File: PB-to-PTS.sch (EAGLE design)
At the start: 4 parts, among them J1 PulseBlaster, J3 PTS-PORT

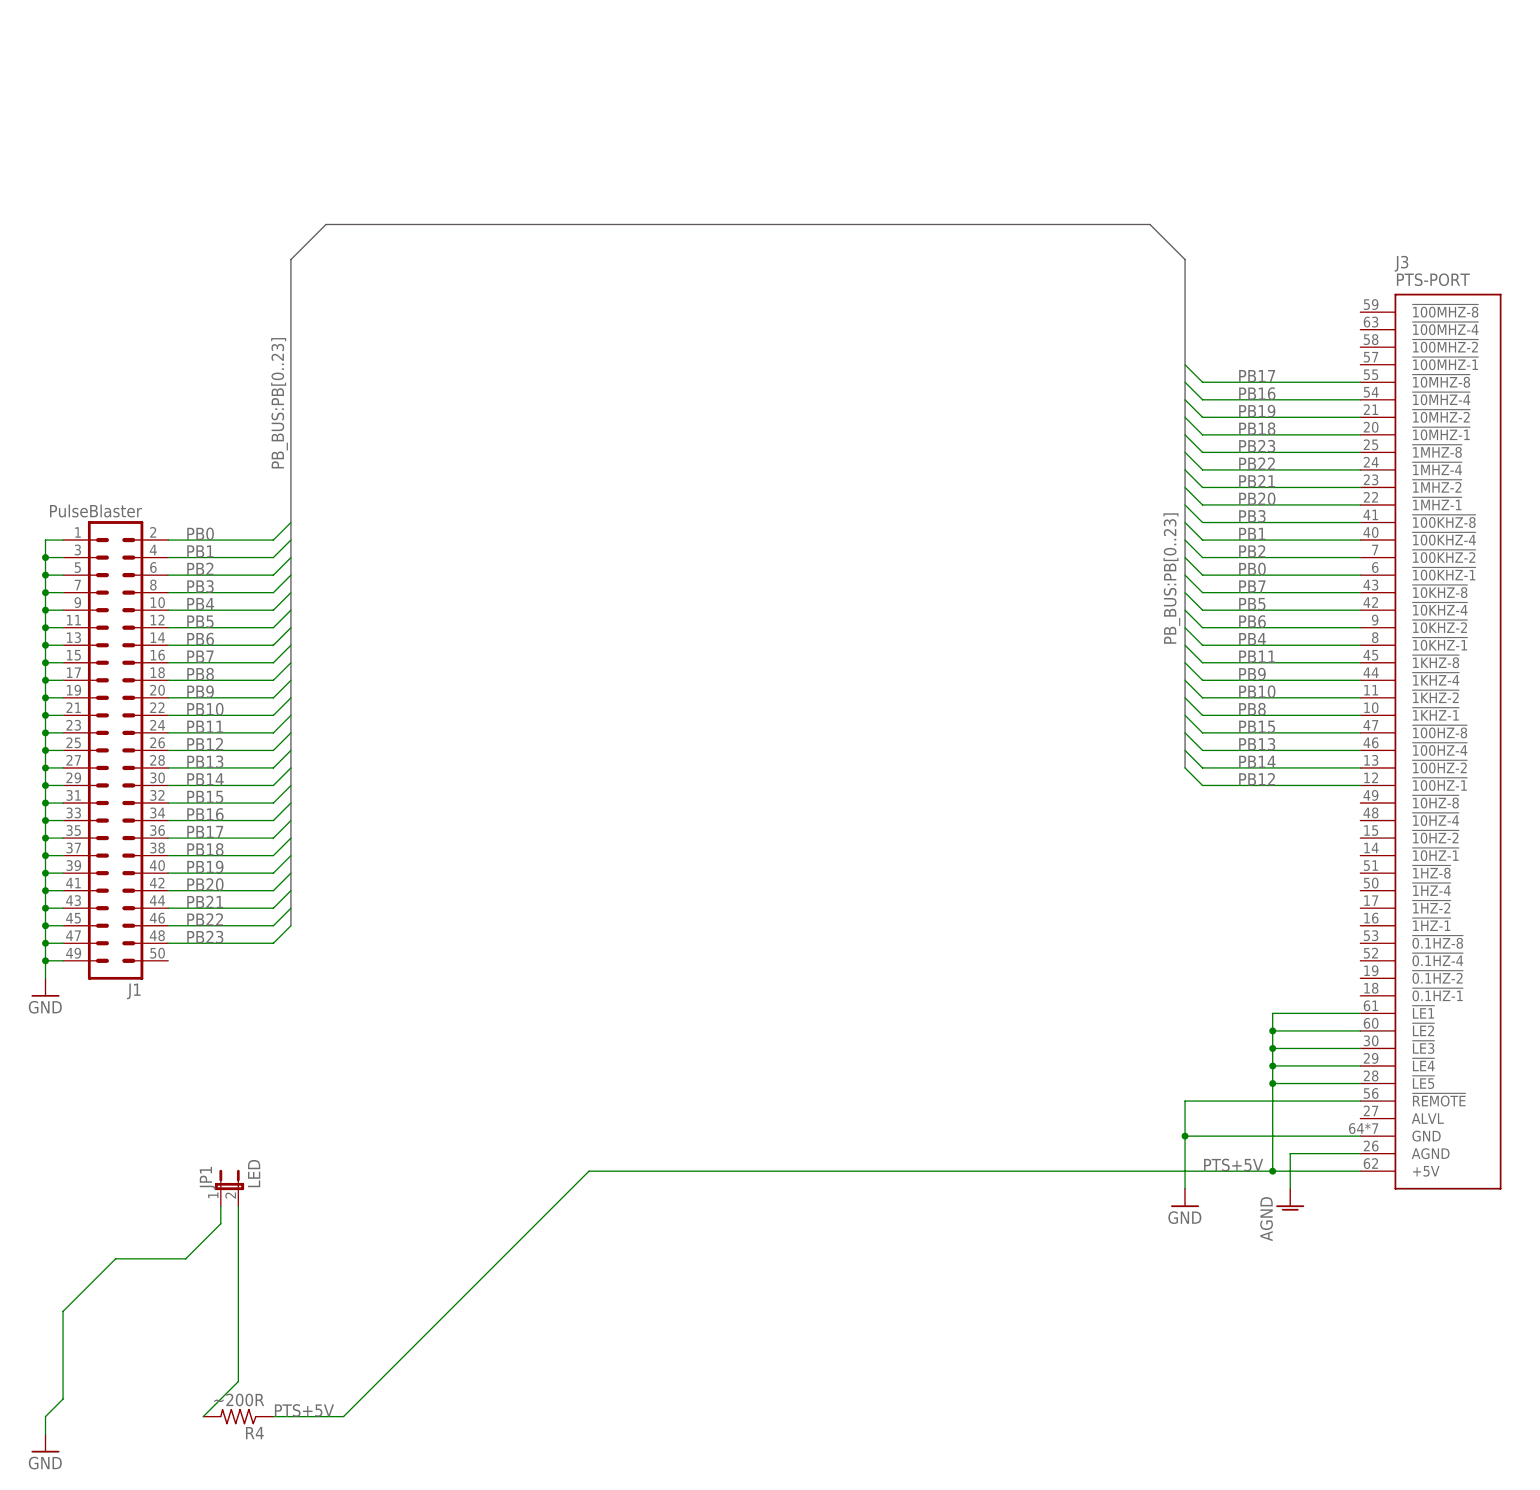
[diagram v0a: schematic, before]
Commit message: Clean up schematic, route board
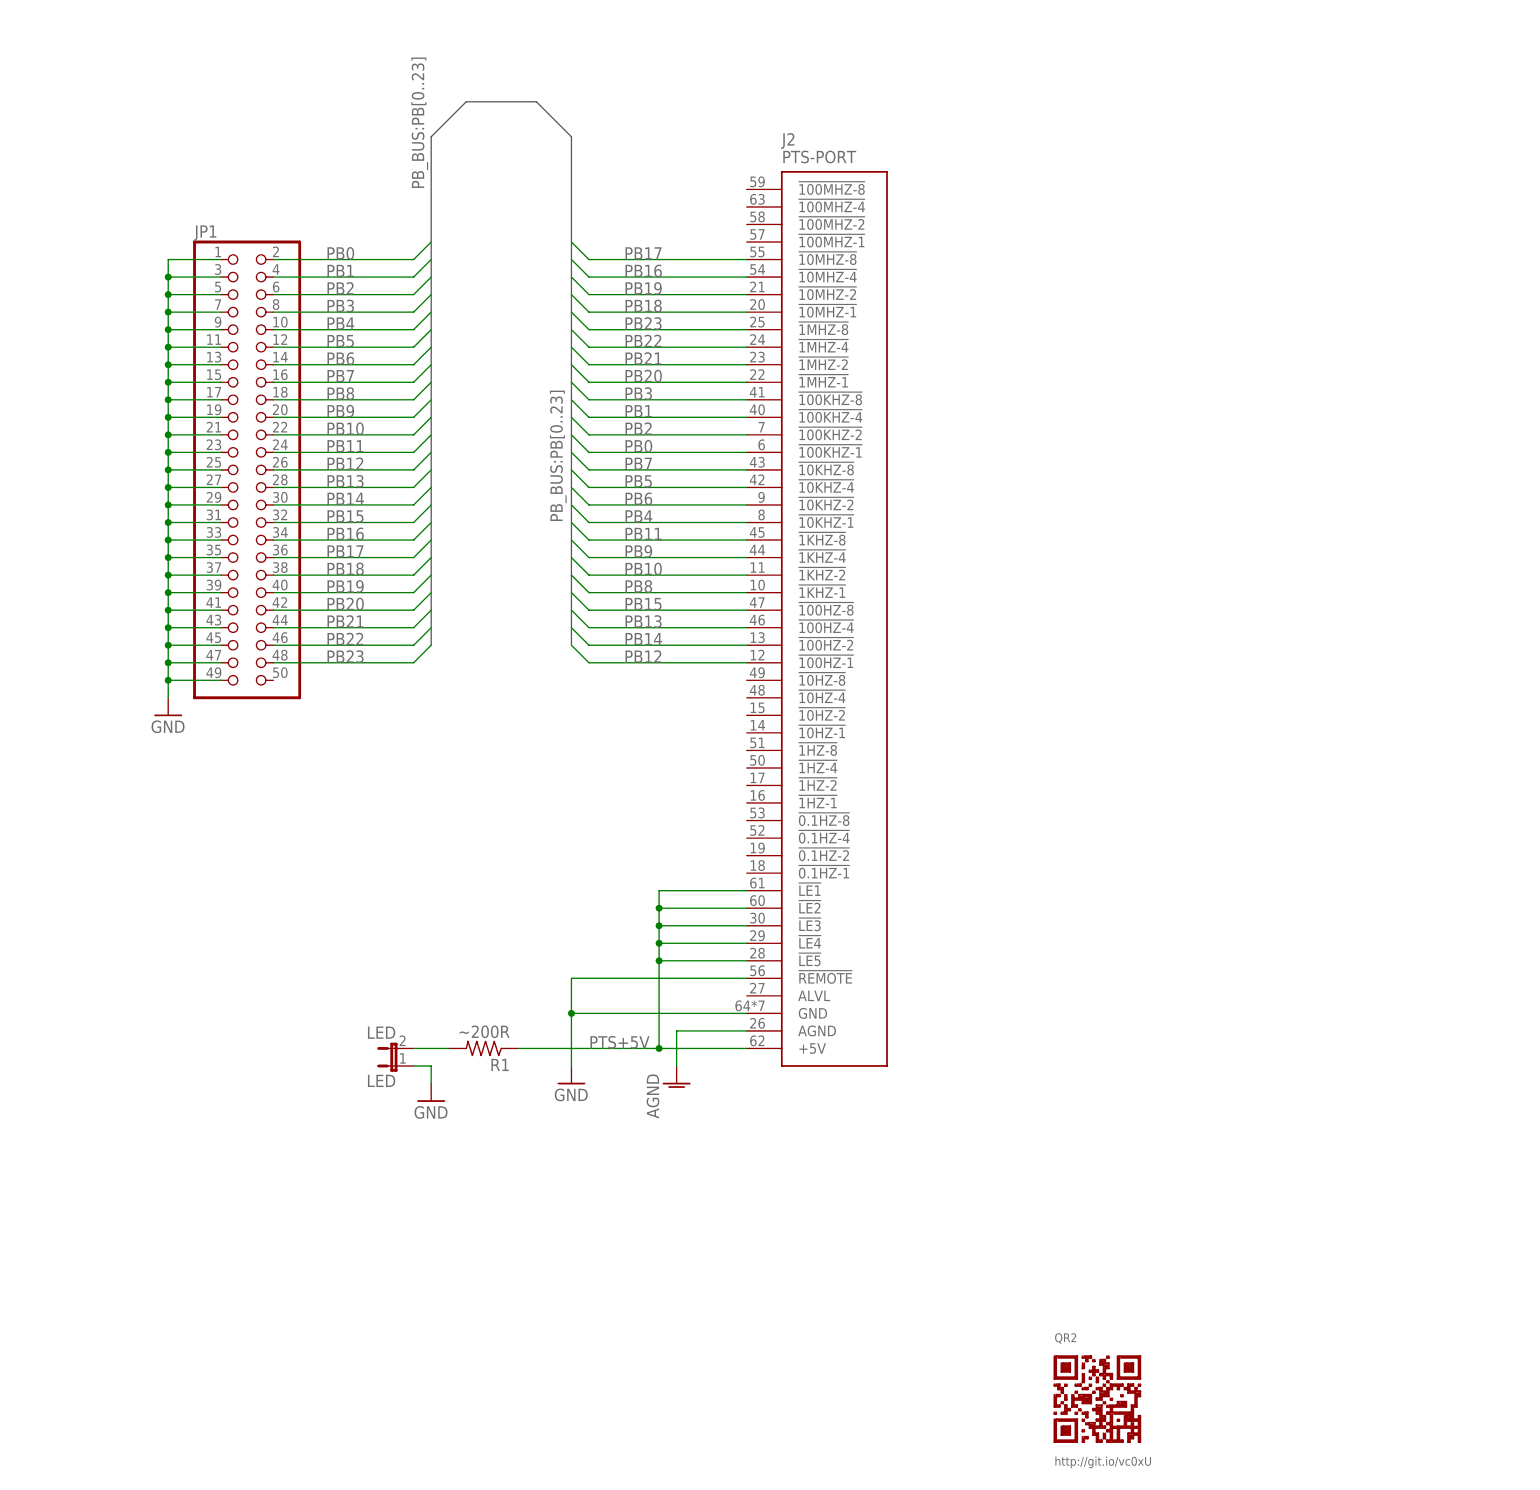
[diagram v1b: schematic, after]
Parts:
- removed J1: PulseBlaster, PTS_Board_Lib:HARTING-09185505909
- removed J3: PTS-PORT, PTS_Board_Lib:PTS-PORT
- removed R4: ~200R, resistor:R-US_R1206
- added J2: PTS-PORT, PTS_Board_Lib:PTS-PORT
- added LED: LED, jumper:JP1E
- added QR2: QR-HTTP://GIT.IO/VC0XU, QR-git.io-vc0xU:QR-HTTP://GIT.IO/VC0XU
- added R1: ~200R, resistor:R-US_R0805
- JP1: value LED -> (none); device jumper:JP1E -> pinhead:PINHD-2X25
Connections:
- net AGND: now also J2.AGND; no longer J3.AGND
- net GND: now also J2.!REMOTE, J2.GND, JP1.11, JP1.13, JP1.15, JP1.17, JP1.19, JP1.21, JP1.23, JP1.25, JP1.27, JP1.29, JP1.3, JP1.31, JP1.33, JP1.35, JP1.37, JP1.39, JP1.41, JP1.43, JP1.45, JP1.47, JP1.49, JP1.5, JP1.7, JP1.9, LED.1; no longer J1.1, J1.11, J1.13, J1.15, J1.17, J1.19, J1.21, J1.23, J1.25, J1.27, J1.29, J1.3, J1.31, J1.33, J1.35, J1.37, J1.39, J1.41, J1.43, J1.45, J1.47, J1.49, J1.5, J1.7, J1.9, J3.!REMOTE, J3.GND
- net N$3: now also LED.2, R1.2; no longer JP1.2, R4.2
- net PB0: now also J2.!100KHZ-1, JP1.2; no longer J1.2, J3.!100KHZ-1
- net PB1: now also J2.!100KHZ-4, JP1.4; no longer J1.4, J3.!100KHZ-4
- net PB10: now also J2.!1KHZ-2, JP1.22; no longer J1.22, J3.!1KHZ-2
- net PB11: now also J2.!1KHZ-8, JP1.24; no longer J1.24, J3.!1KHZ-8
- net PB12: now also J2.!100HZ-1, JP1.26; no longer J1.26, J3.!100HZ-1
- net PB13: now also J2.!100HZ-4, JP1.28; no longer J1.28, J3.!100HZ-4
- net PB14: now also J2.!100HZ-2, JP1.30; no longer J1.30, J3.!100HZ-2
- net PB15: now also J2.!100HZ-8, JP1.32; no longer J1.32, J3.!100HZ-8
- net PB16: now also J2.!10MHZ-4, JP1.34; no longer J1.34, J3.!10MHZ-4
- net PB17: now also J2.!10MHZ-8, JP1.36; no longer J1.36, J3.!10MHZ-8
- net PB18: now also J2.!10MHZ-1, JP1.38; no longer J1.38, J3.!10MHZ-1
- net PB19: now also J2.!10MHZ-2, JP1.40; no longer J1.40, J3.!10MHZ-2
- net PB2: now also J2.!100KHZ-2, JP1.6; no longer J1.6, J3.!100KHZ-2
- net PB20: now also J2.!1MHZ-1, JP1.42; no longer J1.42, J3.!1MHZ-1
- net PB21: now also J2.!1MHZ-2, JP1.44; no longer J1.44, J3.!1MHZ-2
- net PB22: now also J2.!1MHZ-4, JP1.46; no longer J1.46, J3.!1MHZ-4
- net PB23: now also J2.!1MHZ-8, JP1.48; no longer J1.48, J3.!1MHZ-8
- net PB3: now also J2.!100KHZ-8, JP1.8; no longer J1.8, J3.!100KHZ-8
- net PB4: now also J2.!10KHZ-1, JP1.10; no longer J1.10, J3.!10KHZ-1
- net PB5: now also J2.!10KHZ-4, JP1.12; no longer J1.12, J3.!10KHZ-4
- net PB6: now also J2.!10KHZ-2, JP1.14; no longer J1.14, J3.!10KHZ-2
- net PB7: now also J2.!10KHZ-8, JP1.16; no longer J1.16, J3.!10KHZ-8
- net PB8: now also J2.!1KHZ-1, JP1.18; no longer J1.18, J3.!1KHZ-1
- net PB9: now also J2.!1KHZ-4, JP1.20; no longer J1.20, J3.!1KHZ-4
- net PTS+5V: now also J2.!LE1, J2.!LE2, J2.!LE3, J2.!LE4, J2.!LE5, J2.+5V, R1.1; no longer J3.!LE1, J3.!LE2, J3.!LE3, J3.!LE4, J3.!LE5, J3.+5V, R4.1
